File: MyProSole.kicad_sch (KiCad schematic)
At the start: 15 parts, among them J1 Conn_01x07_Socket_XIAO_ESP32C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, J2 XIAO_ESP32C3, J3 i2c-bus, J4 FSR1, J5 FSR2, J6 FSR3, J7 Conn_01x06

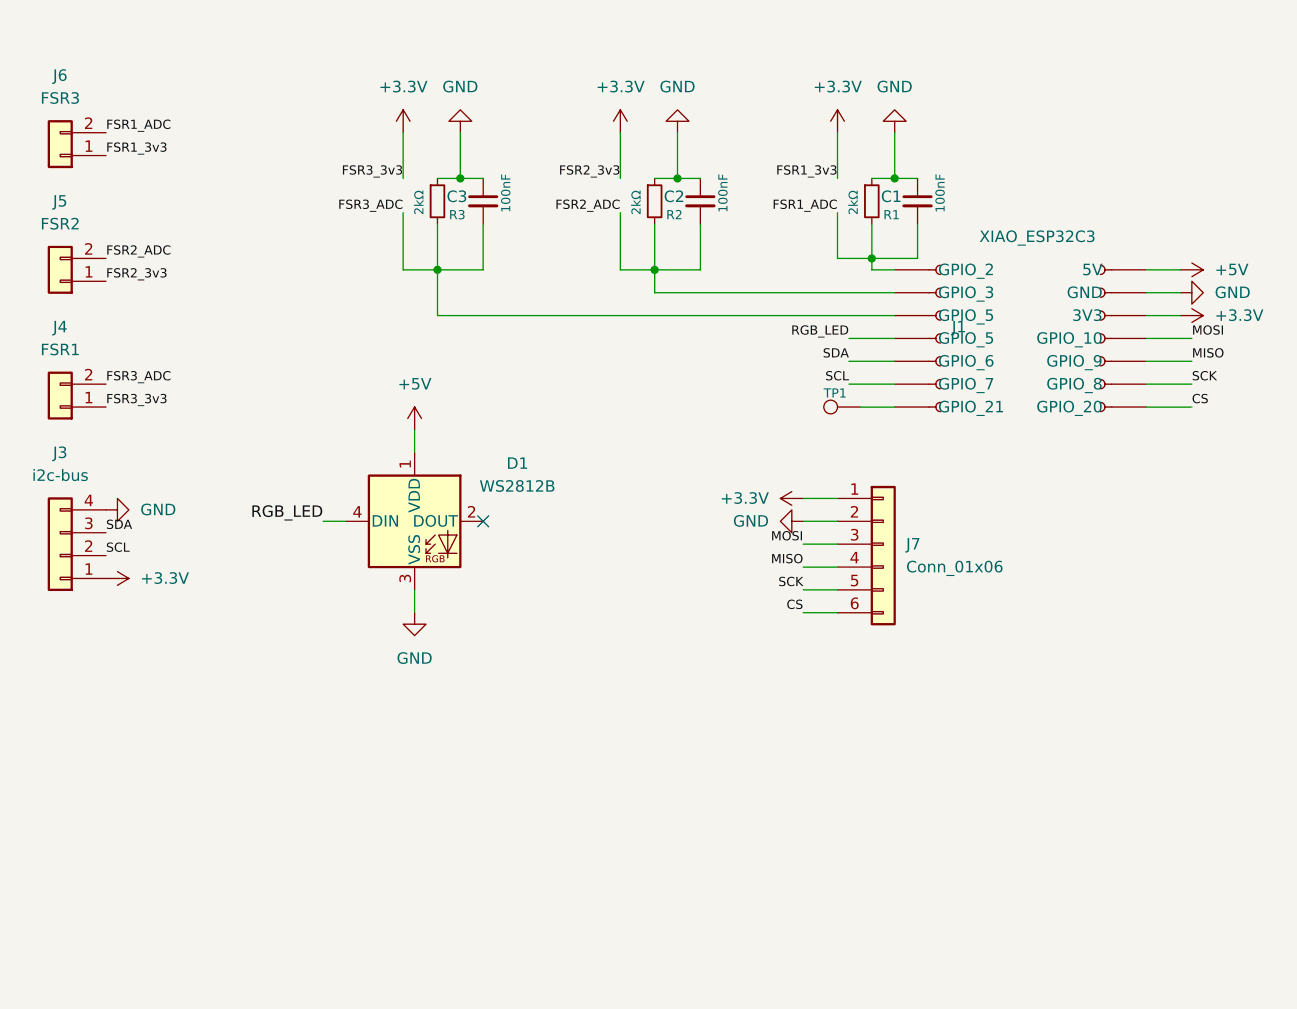
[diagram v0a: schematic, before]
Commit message: Fix ERC
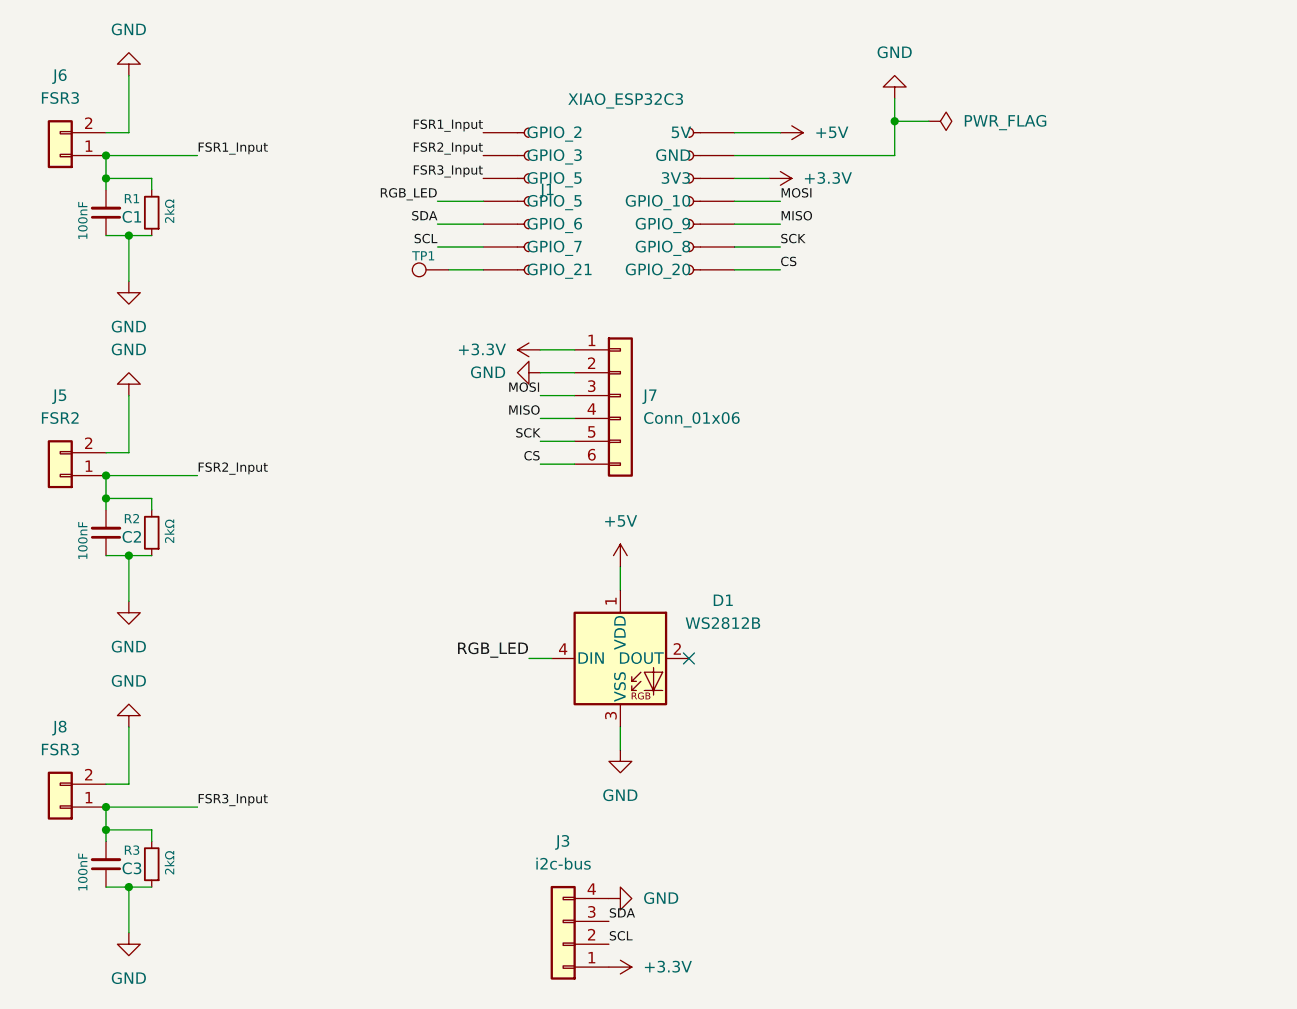
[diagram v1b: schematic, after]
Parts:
- removed J4: FSR1, symbol Connector_Generic:Conn_01x02
- added J8: FSR3, symbol Connector_Generic:Conn_01x02
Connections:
- net +3.3V: no longer J5.1 (Pin_1), J6.1 (Pin_1)
- net GND: now also J5.2 (Pin_2), J6.2 (Pin_2), J8.2 (Pin_2)
- net FSR1_ADC renamed FSR1_Input
- net FSR1_Input: now also J6.1 (Pin_1); no longer J6.2 (Pin_2)
- net FSR2_ADC renamed FSR2_Input
- net FSR2_Input: now also J5.1 (Pin_1); no longer J5.2 (Pin_2)
- net FSR3_ADC renamed FSR3_Input
- net FSR3_Input: now also J8.1 (Pin_1)
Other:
- moved on the sheet: C1, D1, J1, J3, J5, J7, R1, TP1
